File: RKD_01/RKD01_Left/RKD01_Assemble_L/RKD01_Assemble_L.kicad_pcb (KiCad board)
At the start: 2 copper layers, 164.3 x 126.2 mm, 82 parts, among them J1 TRRS, M1 Mark, M10 Mark, M2 Mark, M3 Mark, M4 Mark, M5 Mark, M6 Mark, M7 Mark, M8 Mark, M9 Mark, SW1 SW_Push, SW10 SW_Push, SW11 SW_Push, SW12 SW_Push, SW13 SW_Push, SW14 SW_Push, SW15 SW_Push, SW16 SW_Push, SW17 SW_Push, SW18 SW_Push, SW19 SW_Push, SW2 SW_Push, SW20 SW_Push, SW21 SW_Push, SW22 SW_Push, SW23 SW_Push, SW24 SW_Push, SW25 SW_Push, SW26 SW_Push, SW27 SW_Push, SW28 SW_Push, SW29 SW_Push, SW3 SW_Push, SW30 SW_Push, SW31 SW_Push, SW32 SW_Push, SW33 SW_Push, SW34 SW_Push, SW35 SW_Push, SW4 SW_Push, SW5 SW_Push, SW6 SW_Push, SW7 SW_Push, SW8 SW_Push, SW9 SW_Push, U1 ProMicro

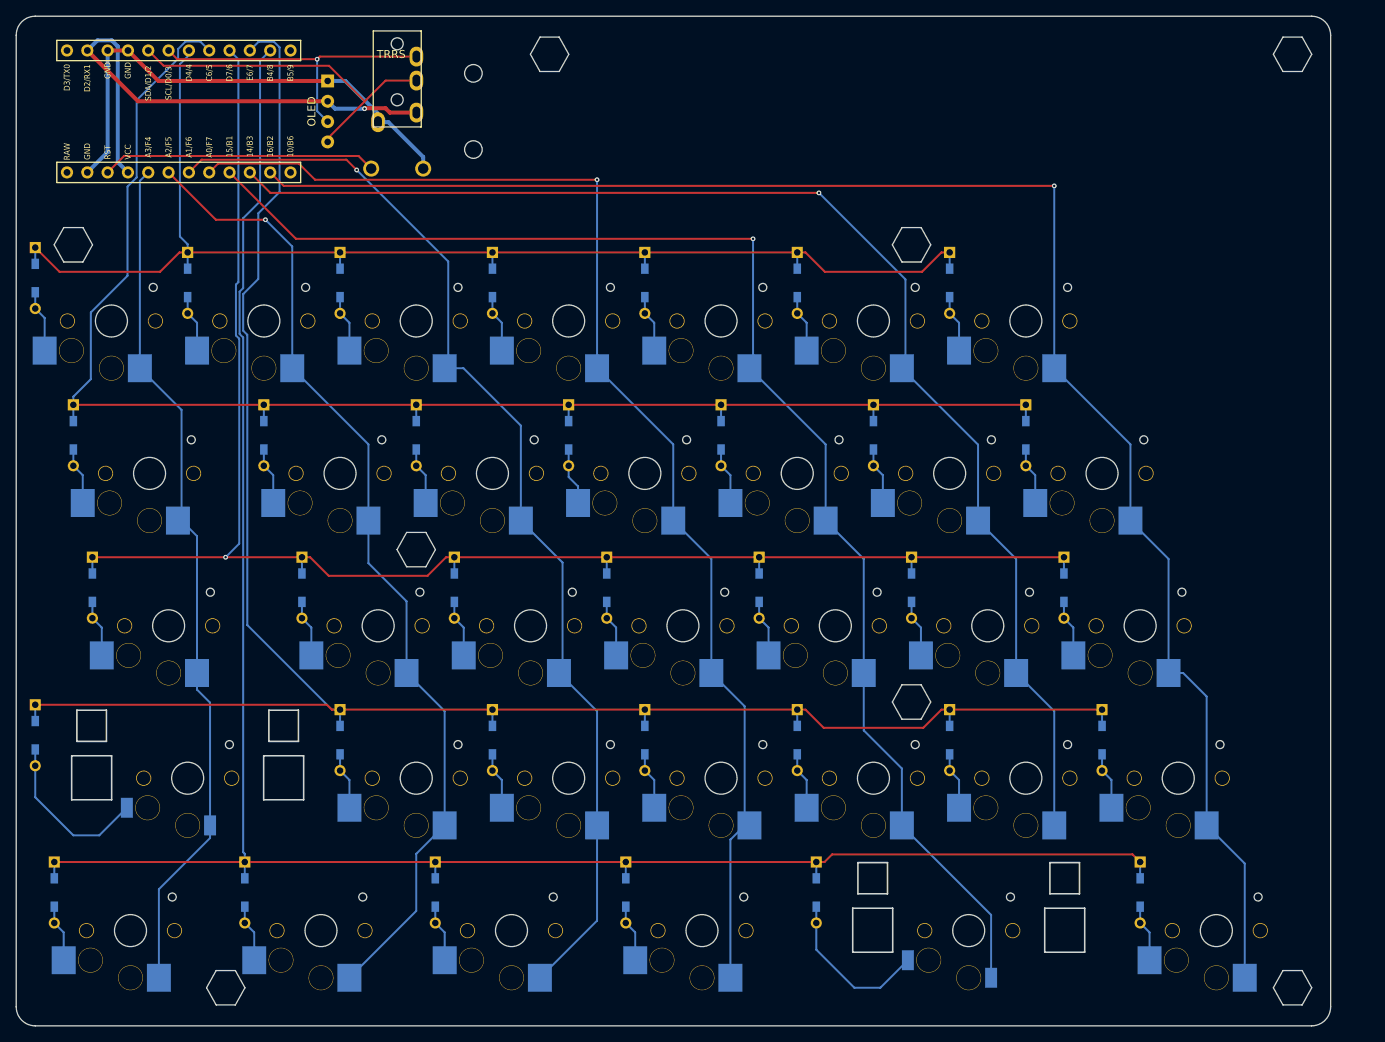
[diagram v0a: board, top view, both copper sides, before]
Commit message: 寸法を見直し
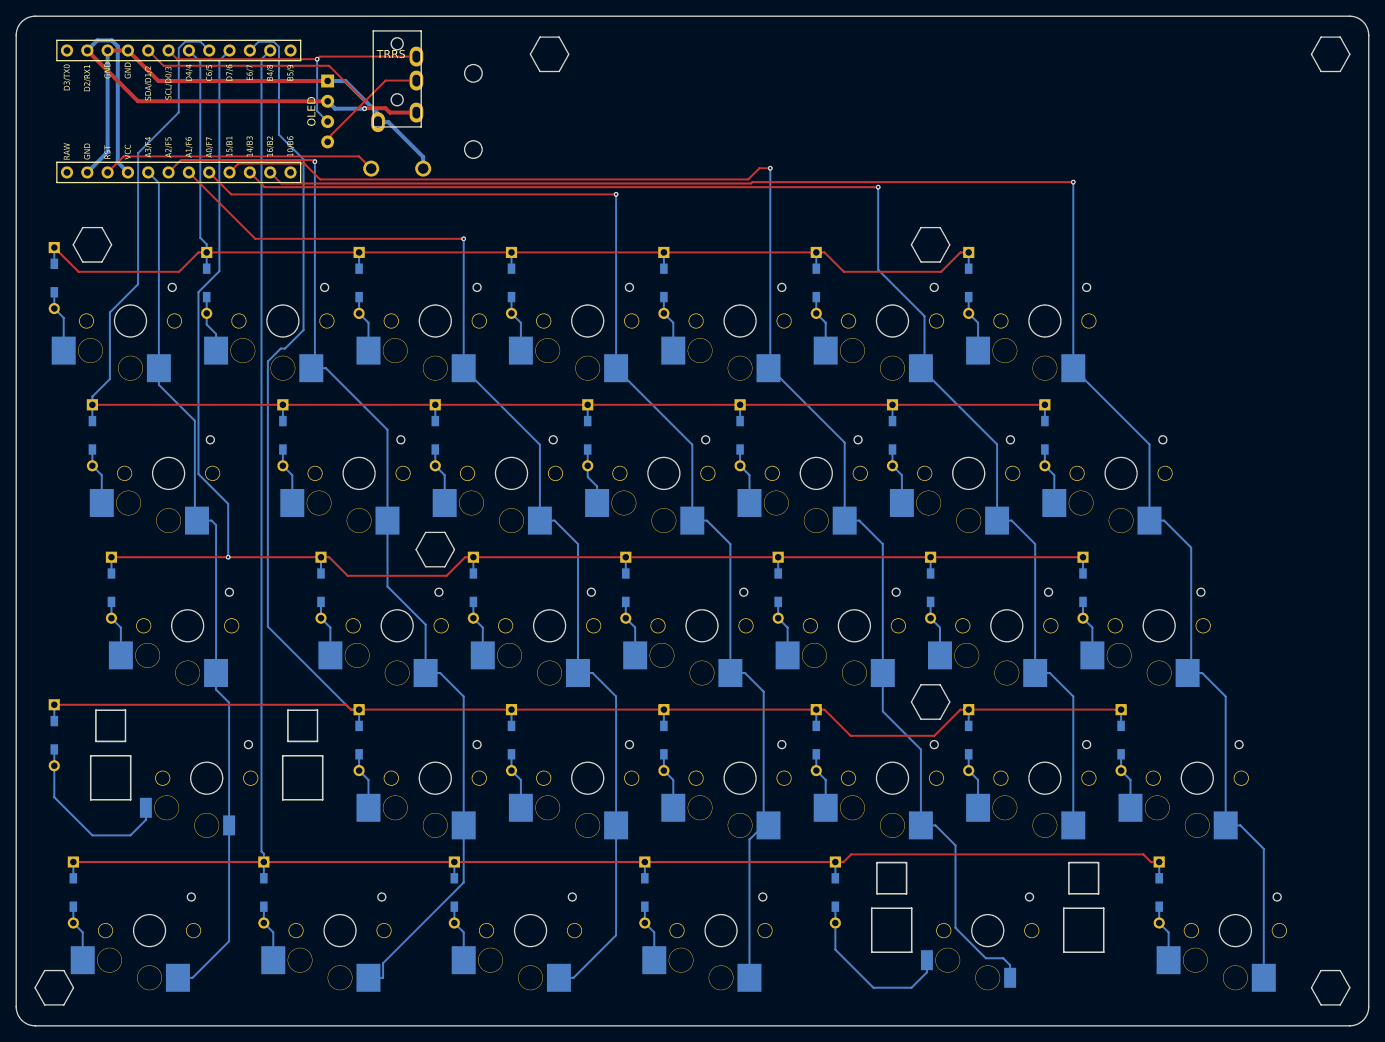
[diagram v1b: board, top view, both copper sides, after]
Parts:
- moved M7 21.4 mm to (26.2, 140.5)
- moved M2 4.76 mm to (185.7, 23.8)
- moved M8 4.76 mm to (185.7, 140.5)
- moved D15 2.38 mm to (76.2, 128.6)
- moved D20 2.38 mm to (100.0, 128.6)
- moved D22 2.38 mm to (111.9, 71.4)
- moved D25 2.38 mm to (123.8, 128.6)
- moved D28 2.38 mm to (135.7, 90.5)
- moved D31 2.38 mm to (150.0, 71.4)
- moved D33 2.38 mm to (159.5, 109.5)
- moved M4 2.38 mm to (135.7, 47.6)
- moved M6 2.38 mm to (135.7, 104.8)
- moved SW13 2.38 mm to (88.1, 95.2)
- moved SW19 2.38 mm to (111.9, 114.3)
- moved SW21 2.38 mm to (111.9, 57.1)
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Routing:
- net Col1: track 123.5 -> 137.1 mm
- net Col4: track 174.2 -> 186.7 mm
- net Col5: track 164.1 -> 172.0 mm
- net Col6: track 208.6 -> 213.8 mm
- net Col2: track 140.7 -> 144.2 mm
- net Col3: track 158.5 -> 161.0 mm
- net Col0: track 107.8 -> 110.0 mm
- net Row3: track 244.5 -> 246.5 mm
- net Row2: track 202.4 -> 204.1 mm
- net Row4: track 252.0 -> 250.7 mm
- net Row1: track 188.0 -> 187.0 mm
- net Net-(D25-A): track 20.2 -> 21.1 mm
- net Net-(D4-A): track 20.8 -> 21.7 mm
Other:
- board size 164.3 x 126.2 mm -> 169.1 x 126.2 mm
